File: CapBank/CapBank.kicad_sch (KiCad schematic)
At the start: 23 parts, among them J1 CONN

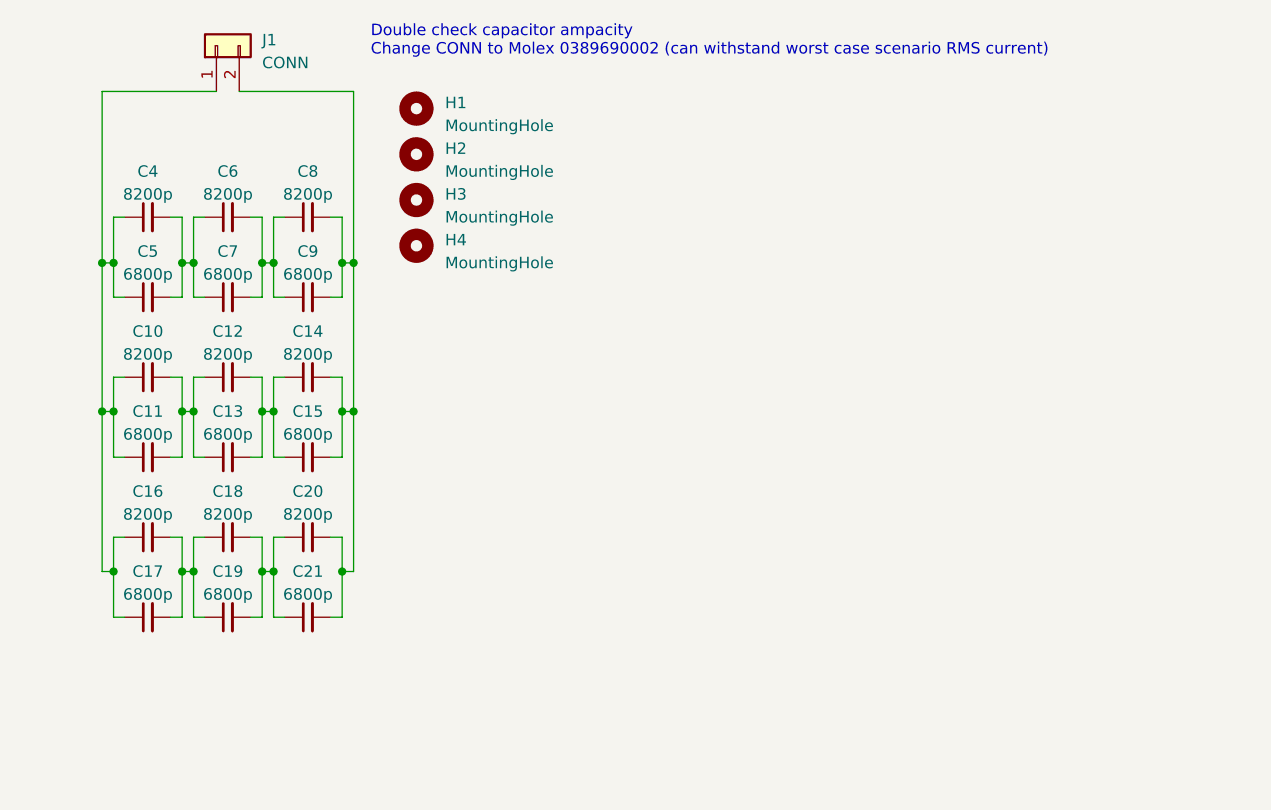
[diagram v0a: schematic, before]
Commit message: Changes to cap bank WIP
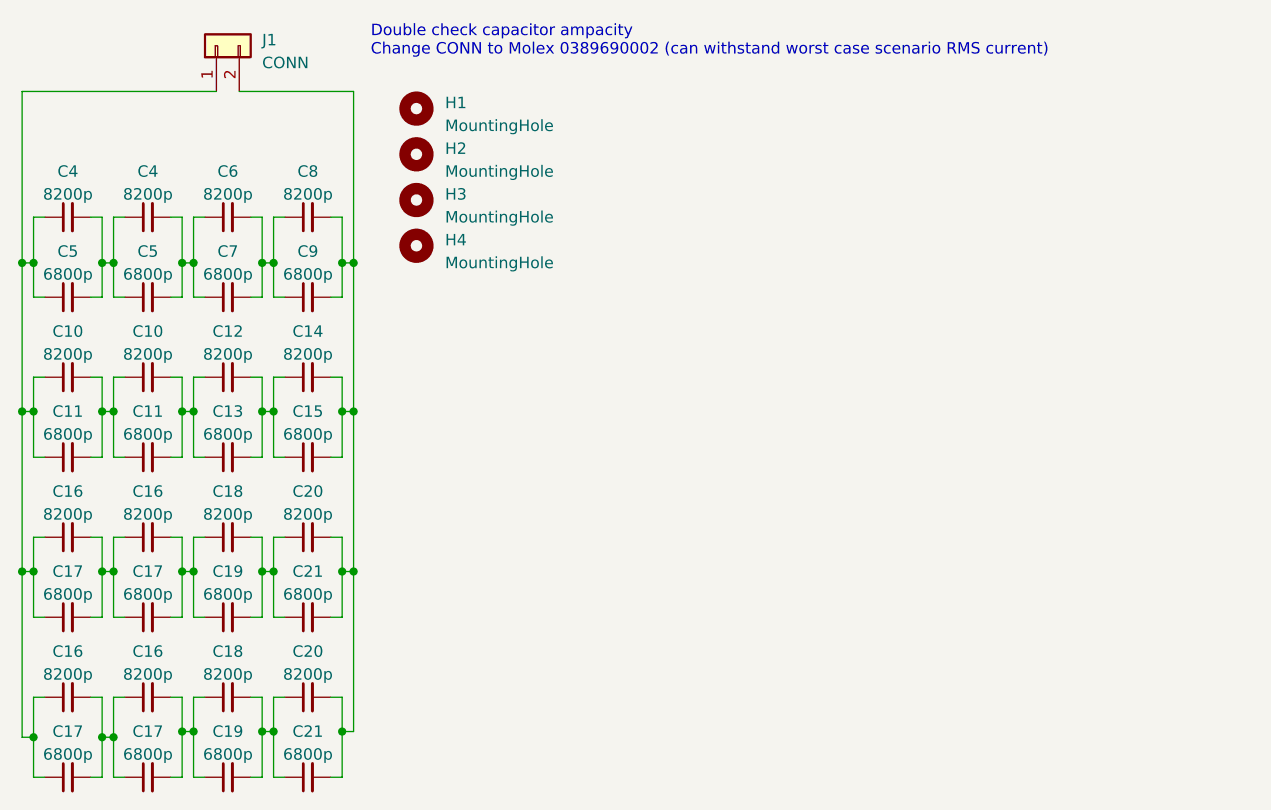
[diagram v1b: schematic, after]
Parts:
- added C10, C16 (x3), C18, C20, C4: 8200p, Capacitor_SMD:C_2220_5650Metric, symbol Device:C_Small
- added C11, C17 (x3), C19, C21, C5: 6800p, Capacitor_SMD:C_2220_5650Metric, symbol Device:C_Small
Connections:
- net at C14.2, C15.2, C20.2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: now also C20.2, C21.2
- new net: C16.2, C17.2, C18.1, C19.1
- new net: C18.2, C19.2, C20.1, C21.1
- new net: C10.1, C11.1, C16.1, C16.1, C17.1, C17.1, C4.1, C5.1, J1.1 (Pin_1)
- new net: C10.1, C10.2, C11.1, C11.2
- new net: C16.1, C16.2, C17.1, C17.2 (x2)
- new net: C4.1, C4.2, C5.1, C5.2
